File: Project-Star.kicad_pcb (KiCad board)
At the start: 4 copper layers, 50 x 50 mm, 35 parts, among them CN1 SC In, CN2 SC Out, Q1 CSD18543Q3A, Q2 CSD18543Q3A, U3 LM25145RGYR, U4 TP Vout, U5 TP Vin, U6 TP GND

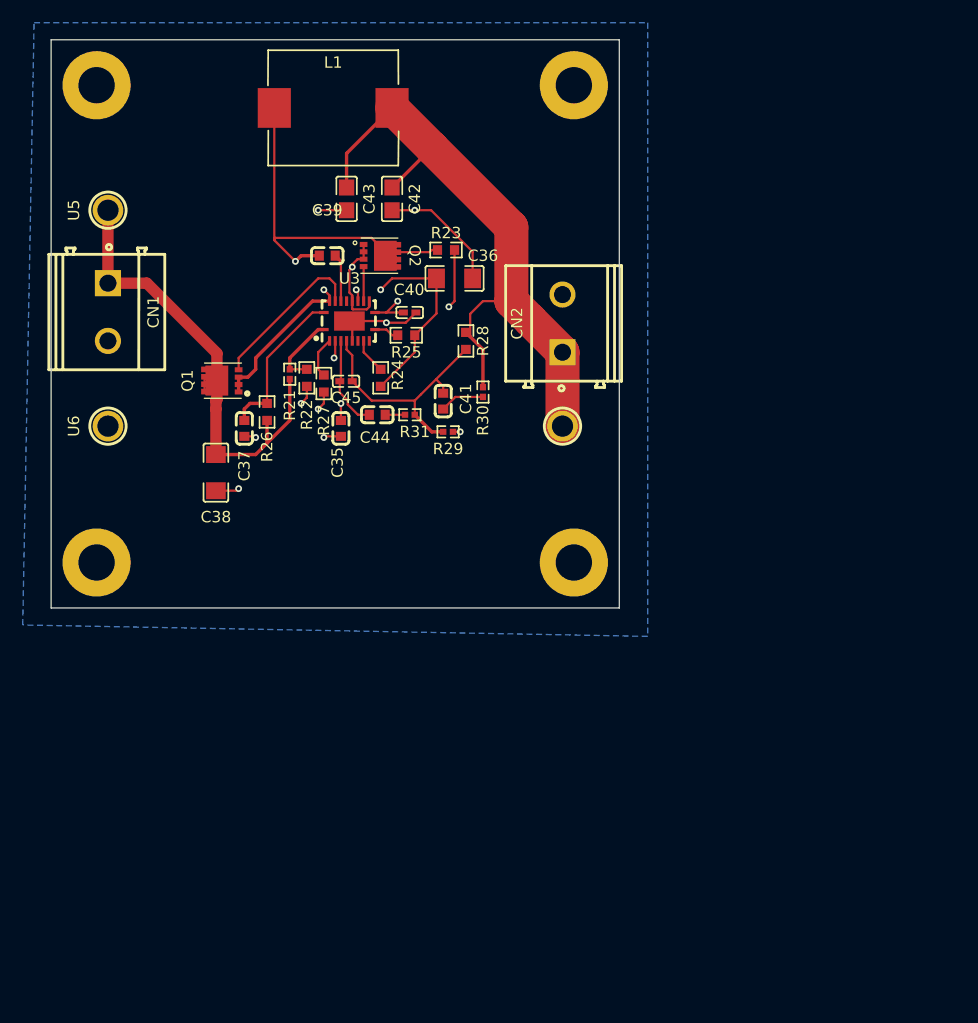
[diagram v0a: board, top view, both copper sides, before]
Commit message: 20V line V2
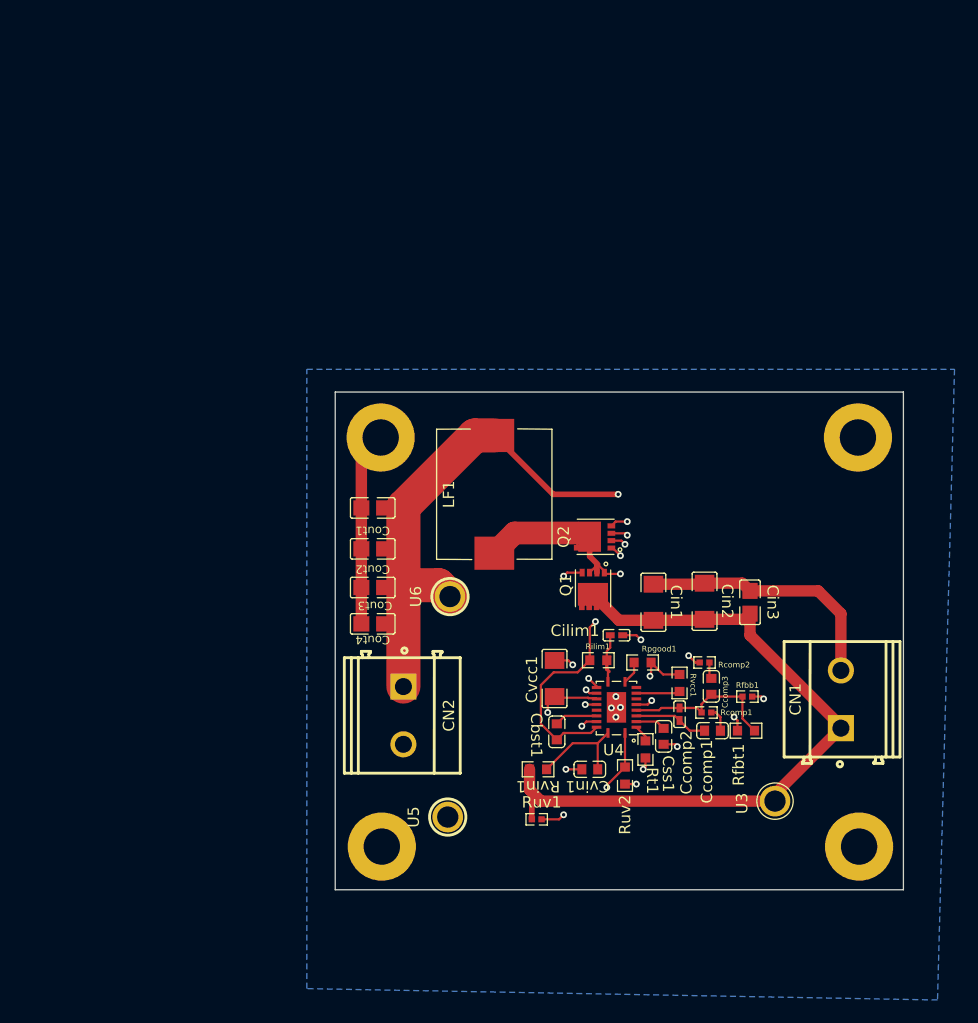
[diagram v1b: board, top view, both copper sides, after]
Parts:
- removed C35: 39n, easyeda2kicad:C0603
- removed C36: 2.2u, easyeda2kicad:C1206
- removed C37, C39: 100n, easyeda2kicad:C0603
- removed C38: 4.7u, easyeda2kicad:C1206
- removed C40: 5.1p, easyeda2kicad:C0402
- removed C41: 390p, easyeda2kicad:C0603
- removed C42, C43: 10u, easyeda2kicad:C0805
- removed C44: 2.7n, easyeda2kicad:C0603
- removed C45: 100p, easyeda2kicad:C0402
- removed L1: 3.3u, easyeda2kicad:IND-SMD_L11.5-W10.0_SMMS1040
- removed R21: 121k, easyeda2kicad:R0402
- removed R22: 8.06k, easyeda2kicad:R0603
- removed R23: 1.33k, easyeda2kicad:R0603
- removed R24, R25: 20k, easyeda2kicad:R0603
- removed R26: 2.1, easyeda2kicad:R0603
- removed R27: 13k, easyeda2kicad:R0603
- removed R28: 18k, easyeda2kicad:R0603
- removed R29: 750, easyeda2kicad:R0402
- removed R30: 16.9, easyeda2kicad:R0402
- removed R31: 3.83k, easyeda2kicad:R0402
- added Cbst1: 100n, easyeda2kicad:C0603, F.Cu at (138.0, 101.9)
- added Ccomp1: 2.7n, easyeda2kicad:C0603, F.Cu at (151.7, 101.8)
- added Ccomp2: 100p, easyeda2kicad:C0402, F.Cu at (148.8, 100.3)
- added Ccomp3: 390p, easyeda2kicad:C0603, F.Cu at (151.6, 97.9)
- added Cilim1: 5.1p, easyeda2kicad:C0402, F.Cu at (143.2, 93.4)
- added Cin1: 4.7u, easyeda2kicad:C1206, F.Cu at (146.5, 90.5)
- added Cin2: 4.7u, easyeda2kicad:C1206, F.Cu at (151.0, 90.4)
- added Cin3: 10u, easyeda2kicad:C0805, F.Cu at (155.0, 90.5)
- added Cout1: 10u, easyeda2kicad:C0805, F.Cu at (121.8, 82.2)
- added Cout2: 10u, easyeda2kicad:C0805, F.Cu at (121.8, 85.8)
- added Cout3: 10u, easyeda2kicad:C0805, F.Cu at (121.8, 89.2)
- added Cout4: 10u, easyeda2kicad:C0805, F.Cu at (121.8, 92.4)
- added Css1: 39n, easyeda2kicad:C0603, F.Cu at (147.4, 102.3)
- added Cvcc1: 2.2u, easyeda2kicad:C1206, F.Cu at (137.8, 97.2)
- added Cvin1: 100n, easyeda2kicad:C0603, F.Cu at (140.9, 105.2)
- added LF1: 3.3u, easyeda2kicad:IND-SMD_L11.5-W10.0_SMMS1040, F.Cu at (132.5, 81.0)
- added Rcomp1: 3.83k, easyeda2kicad:R0402, F.Cu at (151.2, 100.2)
- added Rcomp2: 16.9, easyeda2kicad:R0402, F.Cu at (151.0, 95.8)
- added Rfbb1: 750, easyeda2kicad:R0402, F.Cu at (154.8, 98.8)
- added Rfbt1: 18k, easyeda2kicad:R0603, F.Cu at (154.7, 101.8)
- added Rilim1: 1.33k, easyeda2kicad:R0603, F.Cu at (141.7, 95.6)
- added Rpgood1: 20k, easyeda2kicad:R0603, F.Cu at (145.6, 95.8)
- added Rt1: 13k, easyeda2kicad:R0603, F.Cu at (145.8, 103.5)
- added Ruv1: 121k, easyeda2kicad:R0402, F.Cu at (136.2, 109.6)
- added Ruv2: 8.06k, easyeda2kicad:R0603, F.Cu at (144.0, 105.8)
- added Rvcc1: 20k, easyeda2kicad:R0603, F.Cu at (148.8, 97.6)
- added Rvin1: 2.1, easyeda2kicad:R0603, F.Cu at (136.3, 105.2)
- U3: value LM25145RGYR -> TP Vin; footprint easyeda2kicad:VQFN-20_L4.5-W3.5-P0.50-BL-EP -> easyeda2kicad:TEST-TH_BD3.17-P1.87
- U4: value TP Vout -> LM25145RGYR; footprint easyeda2kicad:TEST-TH_BD3.17-P1.87 -> easyeda2kicad:VQFN-20_L4.5-W3.5-P0.50-BL-EP
- U5: value TP Vin -> TP GND
- U6: value TP GND -> TP Vout
- moved CN1 72.9 mm to (163.0, 99.0), turned to 90 degrees
- moved U5 61.2 mm to (128.4, 109.4)
- moved U3 56.5 mm to (157.2, 108.0)
- moved H1 39.8 mm to (122.5, 76.0)
- moved H2 39.8 mm to (164.5, 76.0)
- moved Q1 37.5 mm to (141.2, 89.4), turned to 180 degrees
- moved CN2 37.2 mm to (124.5, 100.5), turned to -90 degrees
- moved H3 35.4 mm to (164.6, 112.0)
- moved H4 35.4 mm to (122.6, 112.0)
- moved U6 33.6 mm to (128.6, 90.0)
- moved Q2 31.1 mm to (141.3, 84.7), turned to 90 degrees
- moved U4 25.2 mm to (143.2, 99.8)
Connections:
- Q1 pad 1: Net-(U3-SW) -> Net-(U4-SW)
- Q1 pad 2: Net-(U3-SW) -> Net-(U4-SW)
- Q1 pad 3: Net-(U3-SW) -> Net-(U4-SW)
- Q2 pad 5: Net-(U3-SW) -> Net-(U4-SW)
- Q2 pad 6: Net-(U3-SW) -> Net-(U4-SW)
- Q2 pad 7: Net-(U3-SW) -> Net-(U4-SW)
- Q2 pad 8: Net-(U3-SW) -> Net-(U4-SW)
- Q2 pad 9: Net-(U3-SW) -> Net-(U4-SW)
- U3 pad 1: Net-(U3-EN/UVLO) -> /20V_Power_Line/Vin
- U4 pad 1: /20V_Power_Line/Vout -> Net-(U4-EN/UVLO)
- U5 pad 1: /20V_Power_Line/Vin -> GND
- U6 pad 1: GND -> /20V_Power_Line/Vout
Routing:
- net Net-(U3-SW): track 48.3 -> 0.00 mm, vias 2 -> 0
- net Net-(U4-SW): track 0.00 -> 42.0 mm, vias 0 -> 2
- net Net-(U4-VCC): track 0.00 -> 22.7 mm, vias 0 -> 2
- net Net-(U3-FB): track 22.2 -> 0.00 mm
- net /20V_Power_Line/Vin: track 42.9 -> 63.8 mm
- net Net-(U3-VCC): track 20.2 -> 0.00 mm, vias 2 -> 0
- net GND: track 39.0 -> 58.7 mm, vias 10 -> 17
- net Net-(Q2-G): track 3.04 -> 19.5 mm, vias 0 -> 2
- net /20V_Power_Line/Vout: track 59.6 -> 74.1 mm, vias 0 -> 3
- net Net-(U4-FB): track 0.00 -> 14.2 mm
- net Net-(U3-VIN): track 13.9 -> 0.00 mm
- net Net-(U3-ILIM): track 13.8 -> 0.00 mm, vias 2 -> 0
- net Net-(U4-EN/UVLO): track 0.00 -> 12.4 mm, vias 0 -> 2
- net Net-(U4-VIN): track 0.00 -> 9.03 mm
- net Net-(U3-COMP): track 8.20 -> 0.00 mm
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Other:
- board size 50 x 50 mm -> 50 x 43.8 mm
- board text removed: "20k"

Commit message: In Progress v3
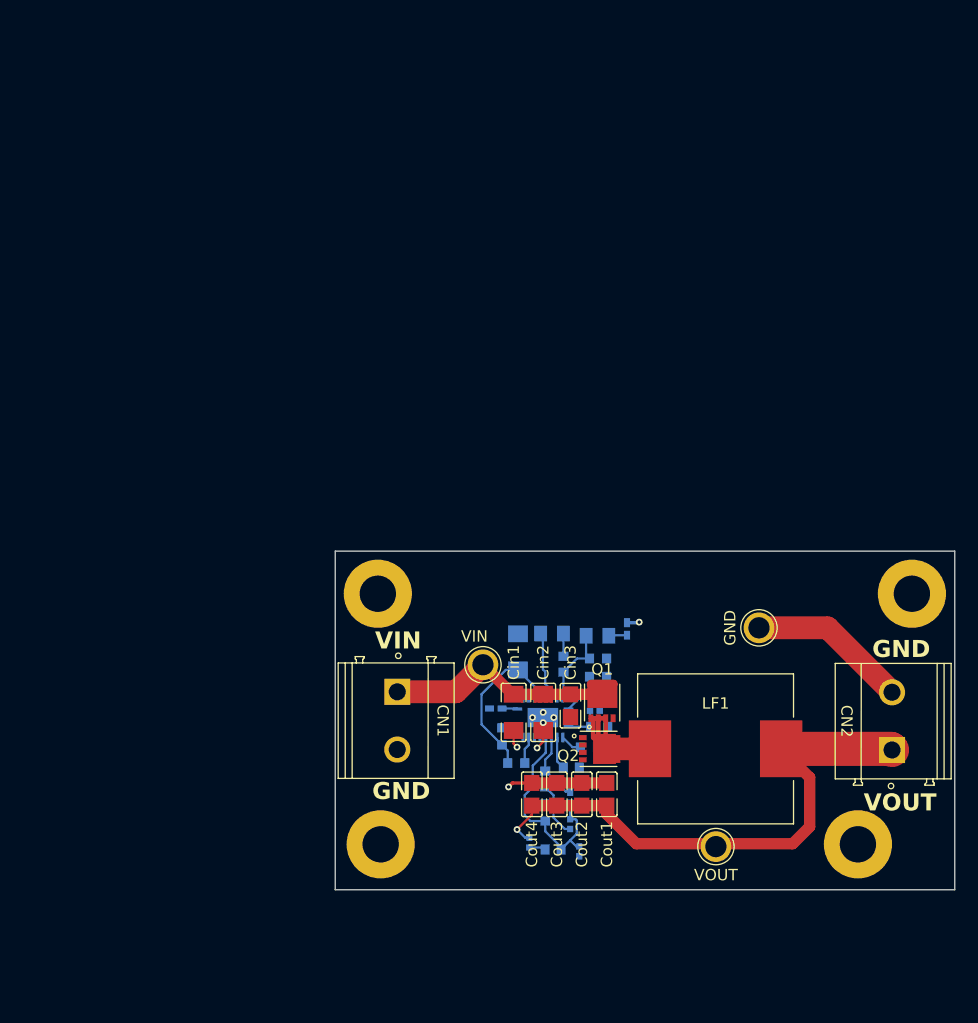
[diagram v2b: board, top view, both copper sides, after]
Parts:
- removed Rfbb1: 750, easyeda2kicad:R0402
- removed Rfbt1: 18k, easyeda2kicad:R0603
- removed Rt1: 13k, easyeda2kicad:R0603
- removed U3: TP Vin, easyeda2kicad:TEST-TH_BD3.17-P1.87
- removed U5: TP GND, easyeda2kicad:TEST-TH_BD3.17-P1.87
- removed U6: TP Vout, easyeda2kicad:TEST-TH_BD3.17-P1.87
- added Csnub1: DNP, easyeda2kicad:C0402, B.Cu at (144.2, 92.8)
- added GND: TP GND, easyeda2kicad:TEST-TH_BD3.17-P1.87, F.Cu at (155.8, 92.8)
- added Rbst1: 4.7, easyeda2kicad:R0805, B.Cu at (137.6, 93.2)
- added Rfb1: 18k, easyeda2kicad:R0603, B.Cu at (137.0, 109.0)
- added Rfb2: 750, easyeda2kicad:R0402, B.Cu at (140.0, 112.4)
- added Rrt1: 13k, easyeda2kicad:R0603, B.Cu at (140.8, 103.2)
- added Rsnub1: DNP, easyeda2kicad:R0805, B.Cu at (141.6, 93.5)
- added VIN: TP Vin, easyeda2kicad:TEST-TH_BD3.17-P1.87, F.Cu at (131.5, 96.0)
- added VOUT: TP Vout, easyeda2kicad:TEST-TH_BD3.17-P1.87, F.Cu at (152.0, 112.0)
- Cbst1, Ccomp1, Ccomp2, Ccomp3, Cilim1, Css1, Cvcc1, Cvin1, Rcomp1, Rcomp2, Rilim1, Rpgood1, Ruv1, Ruv2, Rvcc1, Rvin1, U4: moved to B.Cu
- LF1: footprint easyeda2kicad:IND-SMD_L11.5-W10.0_SMMS1040 -> easyeda2kicad:IND-SMD_L13.8-W12.8
- moved H1 55.2 mm to (164.5, 111.8), turned to 180 degrees
- moved H2 55.2 mm to (122.5, 111.8), turned to 180 degrees
- moved H4 51.7 mm to (169.2, 89.8), turned to 180 degrees
- moved H3 47.8 mm to (122.2, 89.8), turned to 180 degrees
- moved CN2 43.0 mm to (167.5, 101.0), turned to 90 degrees
- moved CN1 39.1 mm to (124.0, 100.9), turned to -90 degrees
- moved Cout1 32.5 mm to (142.4, 107.4), turned to 90 degrees
- moved LF1 29.7 mm to (152.0, 103.4), turned to 0 degrees
- moved Cout2 28.4 mm to (140.2, 107.4), turned to 90 degrees
- moved Cout3 24.4 mm to (138.0, 107.4), turned to 90 degrees
- moved Rcomp2 22.1 mm to (135.6, 111.7), turned to -90 degrees
- moved Cout4 20.5 mm to (135.8, 107.4), turned to 90 degrees
- moved Ccomp3 20.0 mm to (137.7, 112.2), turned to 0 degrees
- moved Q2 18.7 mm to (141.8, 103.4), turned to -90 degrees
- moved Cin3 18.2 mm to (139.2, 99.6), turned to -90 degrees
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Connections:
- Cbst1 pad 2: Net-(U4-BST) -> Net-(Cbst1-Pad2)
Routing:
- net /20V_Power_Line/Vin: track 63.8 -> 22.1 mm
- net GND: track 58.7 -> 33.6 mm, vias 17 -> 8
- net /20V_Power_Line/Vout: track 74.1 -> 52.2 mm, vias 3 -> 1
- net Net-(U4-SW): track 42.0 -> 21.4 mm, vias 2 -> 0
- net Net-(Q2-G): track 19.5 -> 0.00 mm, vias 2 -> 0
- net Net-(Q1-G): track 17.6 -> 0.00 mm, vias 2 -> 0
- net Net-(U4-EN/UVLO): track 12.4 -> 3.40 mm, vias 2 -> 0
- net Net-(U4-VCC): track 22.7 -> 14.1 mm, vias 2 -> 0
- net Net-(U4-FB): track 14.2 -> 19.3 mm
- net Net-(U4-VIN): track 9.03 -> 4.11 mm
- net Net-(U4-ILIM): track 4.77 -> 1.37 mm
- net Net-(Ccomp1-Pad2): track 2.17 -> 4.89 mm
- net Net-(U4-BST): track 3.79 -> 6.04 mm
- net Net-(Cbst1-Pad2): track 0.00 -> 2.00 mm
- net Net-(Csnub1-Pad1): track 0.00 -> 1.62 mm
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- added copper zone on In1.Cu, net GND
- removed copper zone on B.Cu, net GND
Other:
- board size 50 x 43.8 mm -> 54.5 x 29.8 mm
- board text added: "GND"
- board text added: "VIN"
- board text added: "VOUT"
